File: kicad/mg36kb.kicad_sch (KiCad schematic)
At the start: 90 parts, among them SW1 keyswitch, SW10 keyswitch, SW11 keyswitch, SW12 keyswitch, SW13 keyswitch, SW14 keyswitch, SW15 keyswitch, SW16 keyswitch, SW17 keyswitch, SW18 keyswitch, SW19 keyswitch, SW2 keyswitch, SW20 keyswitch, SW21 keyswitch, SW22 keyswitch, SW23 keyswitch, SW24 keyswitch, SW25 keyswitch, SW26 keyswitch, SW27 keyswitch, SW28 keyswitch, SW29 keyswitch, SW3 keyswitch, SW30 keyswitch, SW31 keyswitch, SW32 keyswitch, SW33 keyswitch, SW34 keyswitch, SW35 keyswitch, SW36 keyswitch, SW4 keyswitch, SW5 keyswitch, SW6 keyswitch, SW7 keyswitch, SW8 keyswitch, SW9 keyswitch, U1 Nice_Nano_V2, U2 Nice_Nano_V2

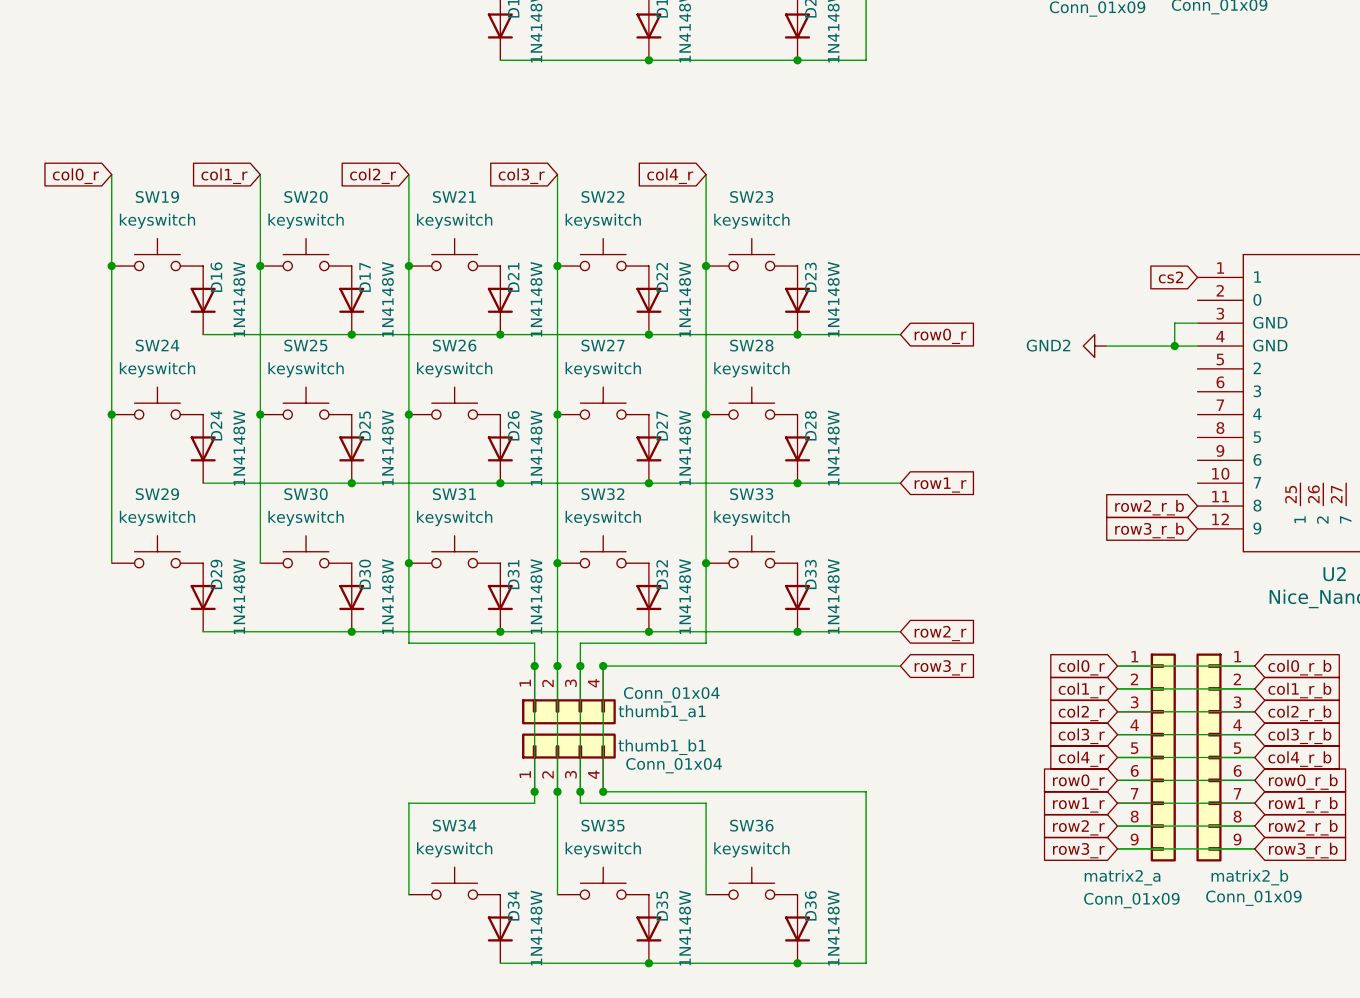
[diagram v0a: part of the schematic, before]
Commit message: init ergogen
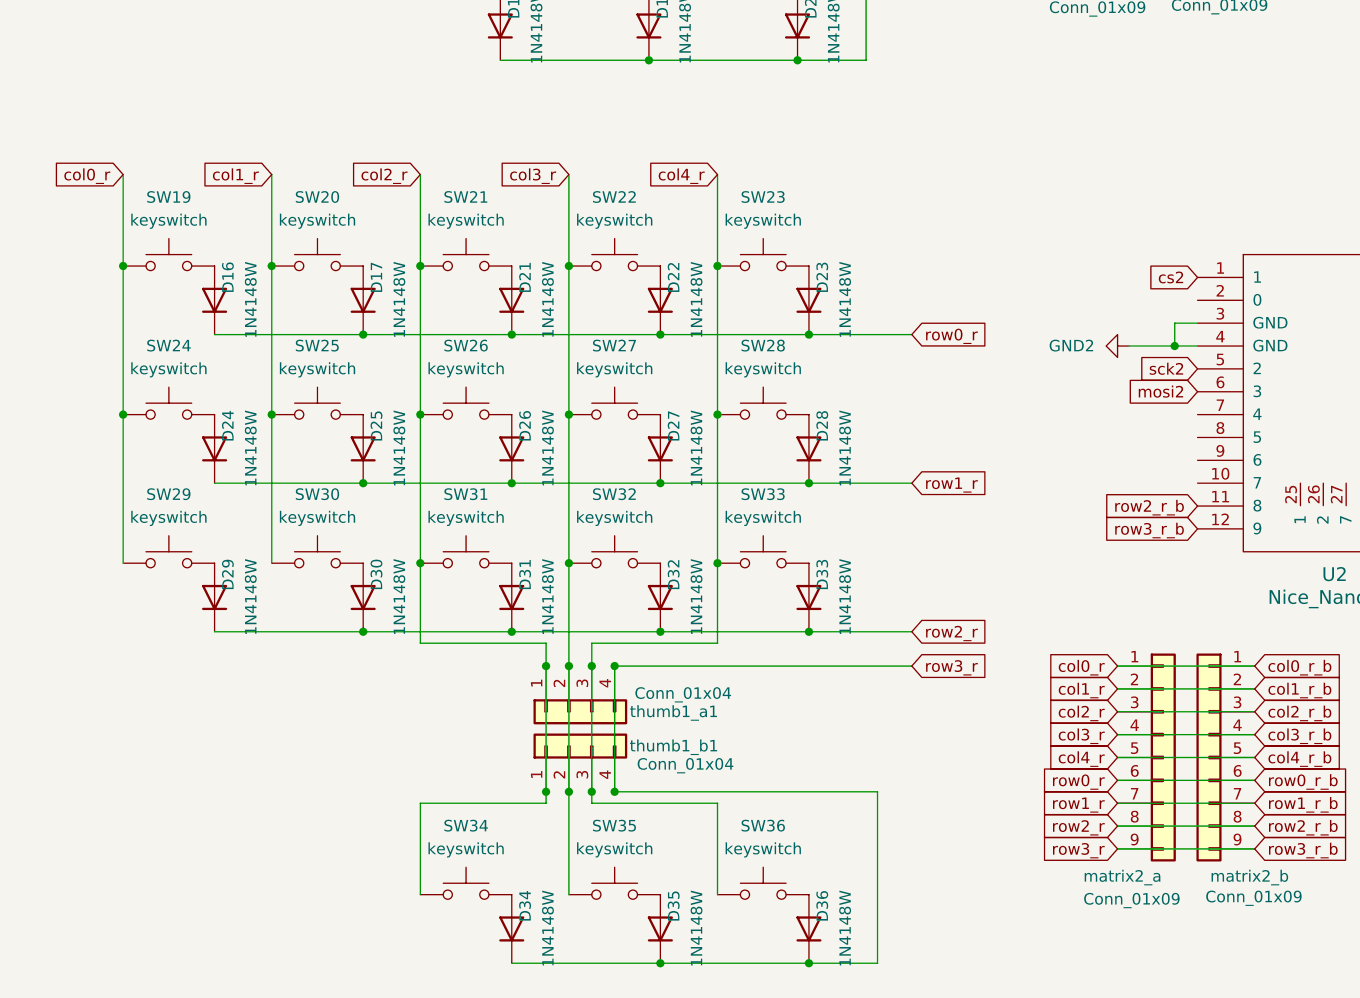
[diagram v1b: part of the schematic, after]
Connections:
- net mosi2: now also U2.6 (3)
- net sck2: now also U2.5 (2)
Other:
- moved on the sheet: D16, D17, D21, D22, D23, D24, D25, D26, D27, D28, D29, D30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
